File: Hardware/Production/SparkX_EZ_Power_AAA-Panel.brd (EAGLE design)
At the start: 187.2 x 136.7 mm, 1236 parts, among them J10 AVR_SPI_PROG_3X2TESTPOINTS, J12 AVR_SPI_PROG_3X2TESTPOINTS, J14 AVR_SPI_PROG_3X2TESTPOINTS, J16 AVR_SPI_PROG_3X2TESTPOINTS, J18 AVR_SPI_PROG_3X2TESTPOINTS, J20 AVR_SPI_PROG_3X2TESTPOINTS, J22 AVR_SPI_PROG_3X2TESTPOINTS, J24 AVR_SPI_PROG_3X2TESTPOINTS, J26 AVR_SPI_PROG_3X2TESTPOINTS, J28 AVR_SPI_PROG_3X2TESTPOINTS, J3 AVR_SPI_PROG_3X2TESTPOINTS, J30 AVR_SPI_PROG_3X2TESTPOINTS, J32 AVR_SPI_PROG_3X2TESTPOINTS, J34 AVR_SPI_PROG_3X2TESTPOINTS, J36 AVR_SPI_PROG_3X2TESTPOINTS, J38 AVR_SPI_PROG_3X2TESTPOINTS, J4 AVR_SPI_PROG_3X2TESTPOINTS, J40 AVR_SPI_PROG_3X2TESTPOINTS, J42 AVR_SPI_PROG_3X2TESTPOINTS, J44 AVR_SPI_PROG_3X2TESTPOINTS, J46 AVR_SPI_PROG_3X2TESTPOINTS, J48 AVR_SPI_PROG_3X2TESTPOINTS, J50 AVR_SPI_PROG_3X2TESTPOINTS, J52 AVR_SPI_PROG_3X2TESTPOINTS, J54 AVR_SPI_PROG_3X2TESTPOINTS, J56 AVR_SPI_PROG_3X2TESTPOINTS, J58 AVR_SPI_PROG_3X2TESTPOINTS, J6 AVR_SPI_PROG_3X2TESTPOINTS, J60 AVR_SPI_PROG_3X2TESTPOINTS, J8 AVR_SPI_PROG_3X2TESTPOINTS, U1 ATTINY43_QFN20, U10 TPS61200, U11 ATTINY43_QFN20, U12 TPS61200, U13 ATTINY43_QFN20, U14 TPS61200, U15 ATTINY43_QFN20, U16 TPS61200, U17 ATTINY43_QFN20, U18 TPS61200, U19 ATTINY43_QFN20, U2 TPS61200, U20 TPS61200, U21 ATTINY43_QFN20, U22 TPS61200, U23 ATTINY43_QFN20, U24 TPS61200, U25 ATTINY43_QFN20, U26 TPS61200, U27 ATTINY43_QFN20, U28 TPS61200, U29 ATTINY43_QFN20, U3 ATTINY43_QFN20, U30 TPS61200, U31 ATTINY43_QFN20, U32 TPS61200, U33 ATTINY43_QFN20, U34 TPS61200, U35 ATTINY43_QFN20, U36 TPS61200, U37 ATTINY43_QFN20, U38 TPS61200, U39 ATTINY43_QFN20, U4 TPS61200, U40 TPS61200, U41 ATTINY43_QFN20, U42 TPS61200, U43 ATTINY43_QFN20, U44 TPS61200, U45 ATTINY43_QFN20, U46 TPS61200, U47 ATTINY43_QFN20, U48 TPS61200, U49 ATTINY43_QFN20, U5 ATTINY43_QFN20, U50 TPS61200, U51 ATTINY43_QFN20, U52 TPS61200, U53 ATTINY43_QFN20, U54 TPS61200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

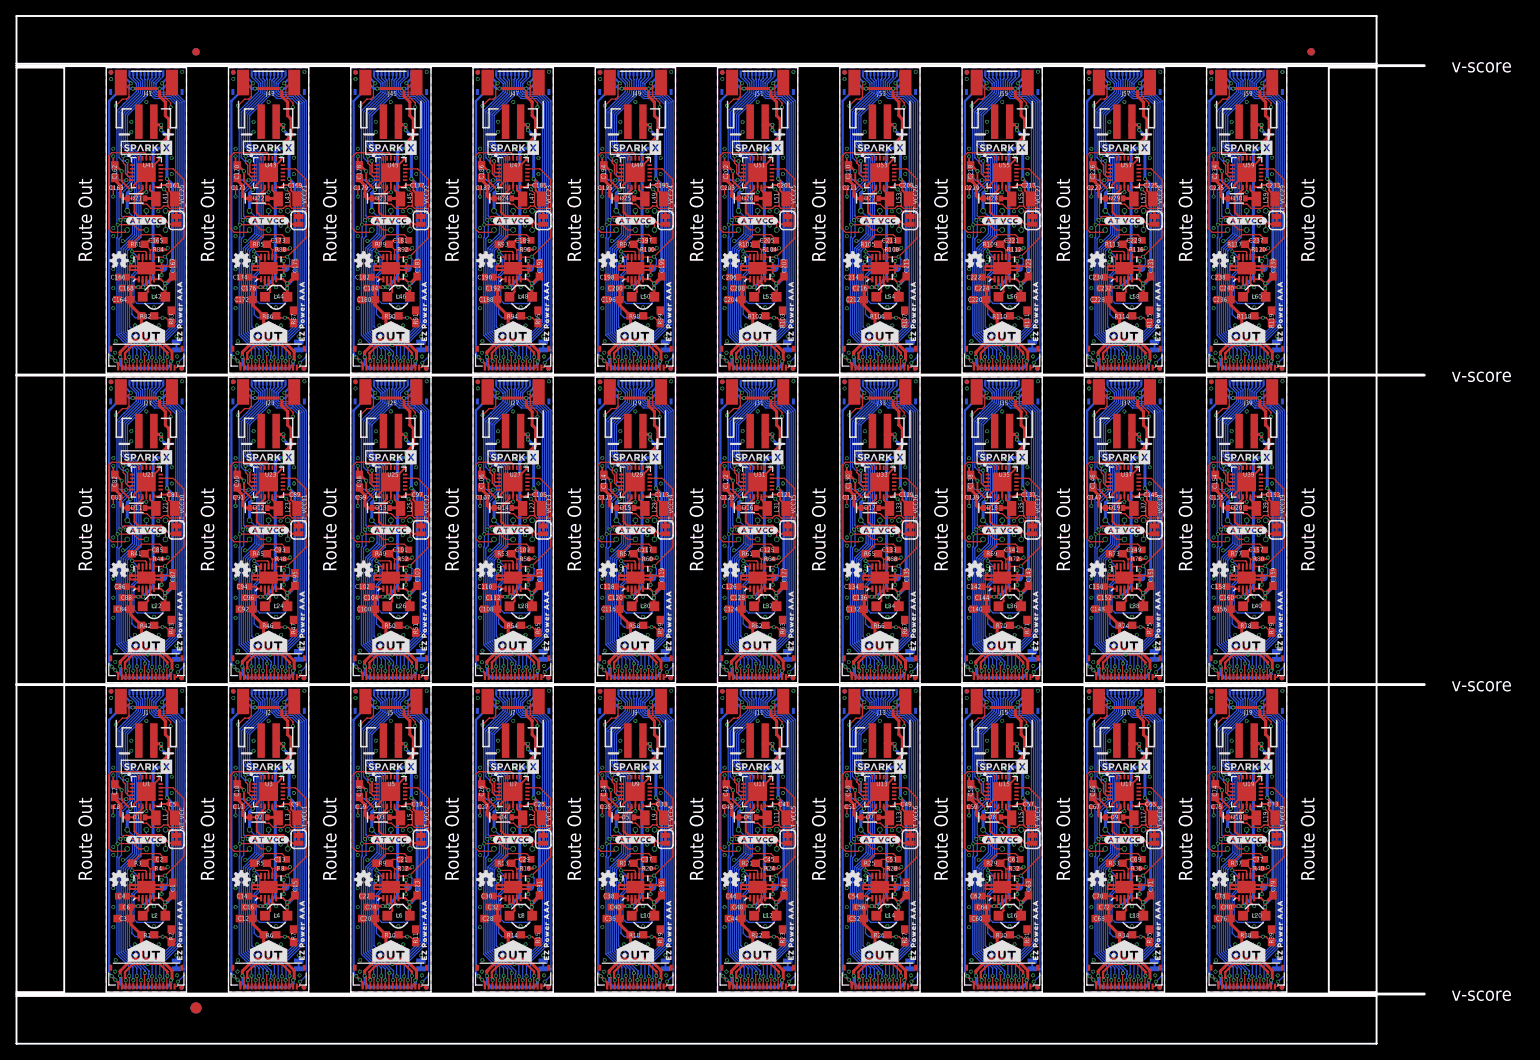
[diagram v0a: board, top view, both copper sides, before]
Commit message: Post-review updates
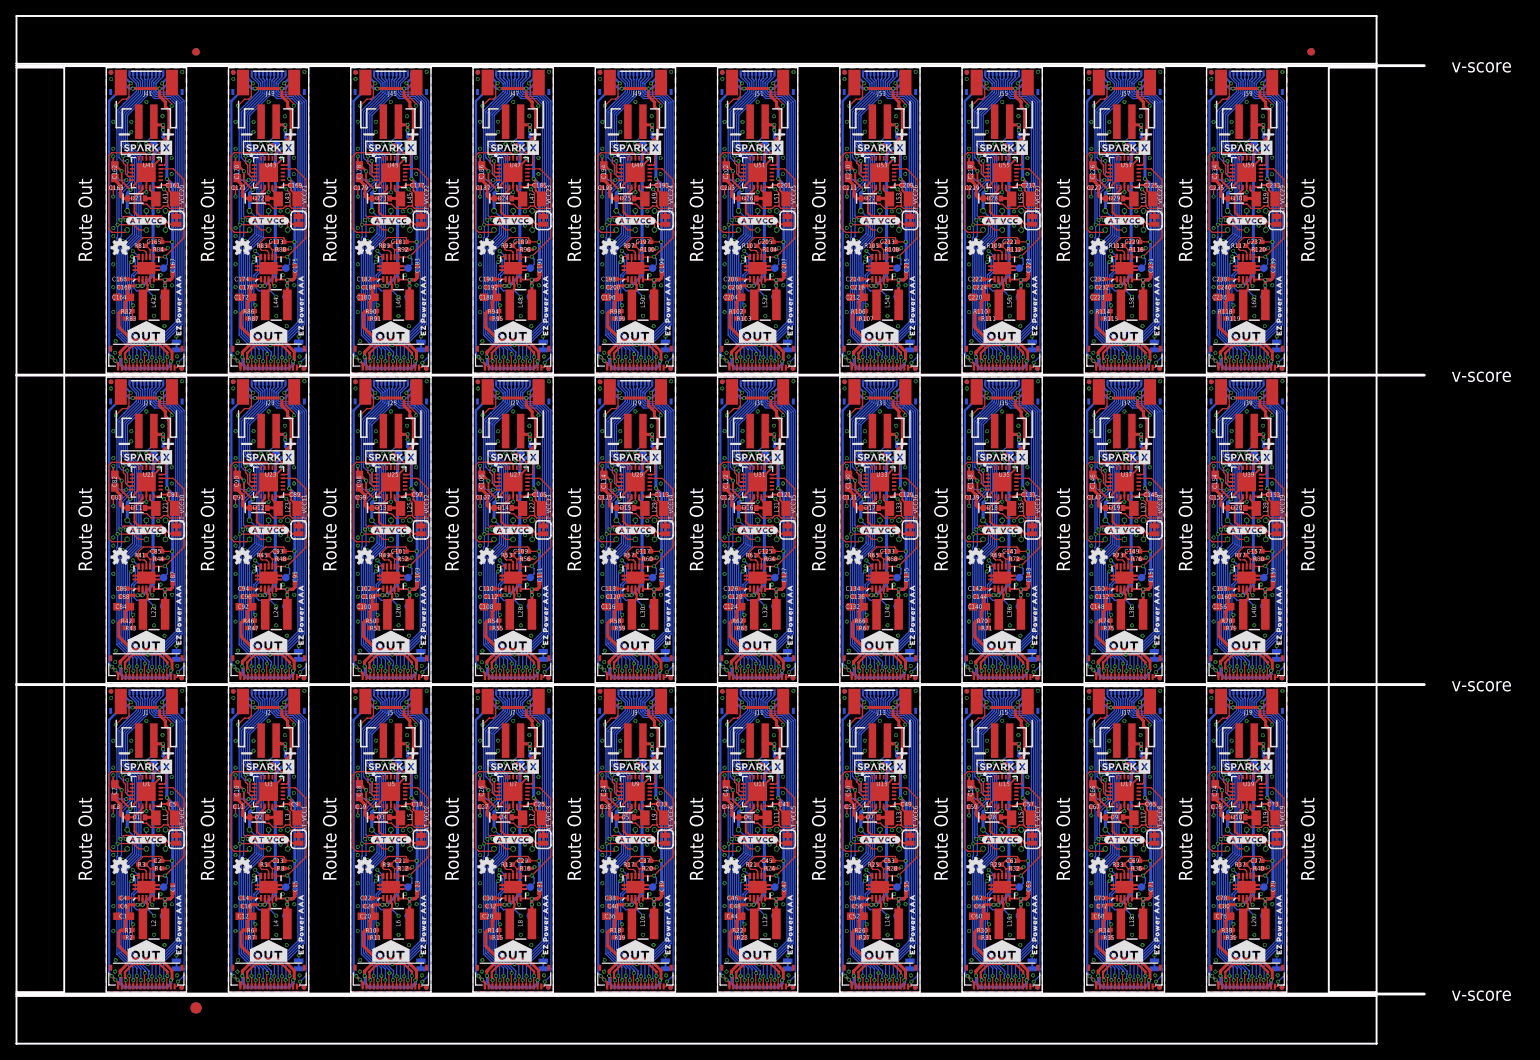
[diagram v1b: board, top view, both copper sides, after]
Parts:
- added RXD, RXD1, RXD10, RXD11, RXD12, RXD13, RXD14, RXD15, RXD16, RXD17, RXD18, RXD19, RXD2, RXD20, RXD21, RXD22, RXD23, RXD24, RXD25, RXD26, RXD27, RXD28, RXD29, RXD3, RXD4, RXD5, RXD6, RXD7, RXD8, RXD9, TXD, TXD1, TXD10, TXD11, TXD12, TXD13, TXD14, TXD15, TXD16, TXD17, TXD18, TXD19, TXD2, TXD20, TXD21, TXD22, TXD23, TXD24, TXD25, TXD26, TXD27, TXD28, TXD29, TXD3, TXD4, TXD5, TXD6, TXD7, TXD8, TXD9: TEST-POINT3X4, SparkFun-Connectors:PAD.03X.04
- added U$301, U$303, U$313, U$315, U$325, U$327, U$337, U$339, U$349, U$351: SPARKX-LOGO3, SparkX:SPARKX-SMALL
- added U$302, U$314, U$326, U$338, U$350: (no value), output:#OUT#0
- added U$304, U$316, U$328, U$340, U$352: (no value), output:#IN#0
- added U$305, U$317, U$329, U$341, U$353: (no value), output:#VIN#0
- added U$306, U$318, U$330, U$342, U$354: (no value), output:#3V3_EN#0
- added U$307, U$319, U$331, U$343, U$355: (no value), output:#PROC_PWR#0
- added U$308, U$320, U$332, U$344, U$356: (no value), output:#AT_VCC#0
- added U$309, U$310, U$321, U$322, U$333, U$334, U$345, U$346, U$357, U$358: (no value), output:EZ_POWER_AAA0
- added U$311, U$323, U$335, U$347, U$359: (no value), output:#TXD#0
- added U$312, U$324, U$336, U$348, U$360: (no value), output:#RXD#0
- C1, C103, C111, C119, C127, C135, C143, C15, C151, C159, C167, C175, C183, C191, C199, C207, C215, C223, C23, C231, C239, C31, C39, C47, C55, C63, C71, C79, C87, C95: device SparkFun-Capacitors:0603 -> SparkFun-Capacitors:0402-TIGHT
- C101, C102, C104, C109, C110, C112, C117, C118, C120, C125, C126, C128, C13, C133, C134, C136, C14, C141, C142, C144, C149, C150, C152, C157, C158, C16, C160, C165, C166, C168, C173, C174, C176, C181, C182, C184, C189, C190, C192, C197, C198, C2, C200, C205, C206, C208, C21, C213, C214, C216, C22, C221, C222, C224, C229, C230, C232, C237, C238, C24, C240, C29, C30, C32, C37, C38, C4, C40, C45, C46, C48, C53, C54, C56, C6, C61, C62, C64, C69, C70, C72, C77, C78, C80, C85, C86, C88, C93, C94, C96: device SparkFun-Capacitors:0402 -> SparkFun-Capacitors:0402-TIGHT
- L10, L12, L14, L16, L18, L2, L20, L22, L24, L26, L28, L30, L32, L34, L36, L38, L4, L40, L42, L44, L46, L48, L50, L52, L54, L56, L58, L6, L60, L8: value 4.7uH, 1.2A -> 4.7μH; device SparkFun:CDRH2D09 -> SparkFun-Coils:INDUCTOR_4X4MM
- R1, R10, R101, R102, R103, R105, R106, R107, R109, R11, R110, R111, R113, R114, R115, R117, R118, R119, R13, R14, R15, R17, R18, R19, R2, R21, R22, R23, R25, R26, R27, R29, R3, R30, R31, R33, R34, R35, R37, R38, R39, R41, R42, R43, R45, R46, R47, R49, R5, R50, R51, R53, R54, R55, R57, R58, R59, R6, R61, R62, R63, R65, R66, R67, R69, R7, R70, R71, R73, R74, R75, R77, R78, R79, R81, R82, R83, R85, R86, R87, R89, R9, R90, R91, R93, R94, R95, R97, R98, R99: device SparkFun-Resistors:0603 -> New-Parts_SparkFun-Resistors:0402-TIGHT
- U$100, U$160, U$220, U$280, U$40: device output:EZ_POWER_AAA0 -> output:#IN#0
- U$101, U$113, U$161, U$173, U$221, U$233, U$281, U$293, U$41, U$53: value SPARKX-LOGO3 -> (none); device SparkX:SPARKX-SMALL -> output:#VIN#0
- U$102, U$162, U$222, U$282, U$42: device output:#OUT#0 -> output:#3V3_EN#0
- U$103, U$151, U$163, U$211, U$223, U$271, U$283, U$31, U$43, U$91: value SPARKX-LOGO3 -> (none); device SparkX:SPARKX-SMALL -> output:#PROC_PWR#0
- U$104, U$164, U$224, U$284, U$44: device output:#IN#0 -> output:#AT_VCC#0
- U$105, U$165, U$225, U$285, U$45: device output:#VIN#0 -> output:EZ_POWER_AAA0
- U$106, U$166, U$226, U$286, U$46: device output:#3V3_EN#0 -> output:EZ_POWER_AAA0
- U$107, U$167, U$227, U$287, U$47: device output:#PROC_PWR#0 -> output:#TXD#0
- U$108, U$168, U$228, U$288, U$48: device output:#AT_VCC#0 -> output:#RXD#0
- U$109, U$159, U$169, U$219, U$229, U$279, U$289, U$39, U$49, U$99: value (none) -> SPARKX-LOGO3; device output:EZ_POWER_AAA0 -> SparkX:SPARKX-SMALL
- U$11, U$134, U$194, U$254, U$74: device output:#IN#0 -> output:#OUT#0
- U$110, U$170, U$230, U$290, U$50: device output:EZ_POWER_AAA0 -> output:#OUT#0
- U$112, U$172, U$232, U$292, U$52: device output:#OUT#0 -> output:#IN#0
- U$114, U$174, U$234, U$294, U$54: device output:#IN#0 -> output:#3V3_EN#0
- U$115, U$175, U$235, U$295, U$55: device output:#VIN#0 -> output:#PROC_PWR#0
- U$116, U$176, U$236, U$296, U$56: device output:#3V3_EN#0 -> output:#AT_VCC#0
- U$117, U$177, U$237, U$297, U$57: device output:#PROC_PWR#0 -> output:EZ_POWER_AAA0
- U$118, U$178, U$238, U$298, U$58: device output:#AT_VCC#0 -> output:EZ_POWER_AAA0
- U$119, U$179, U$239, U$299, U$59: device output:EZ_POWER_AAA0 -> output:#TXD#0
- U$120, U$180, U$240, U$300, U$60: device output:EZ_POWER_AAA0 -> output:#RXD#0
- U$131, U$143, U$191, U$203, U$23, U$251, U$263, U$4, U$71, U$83: value SPARKX-LOGO3 -> (none); device SparkX:SPARKX-SMALL -> output:#TXD#0
- U$132, U$192, U$252, U$72, U$9: device output:#OUT#0 -> output:#RXD#0
- U$135, U$14, U$145, U$195, U$205, U$25, U$255, U$265, U$75, U$85: value (none) -> SPARKX-LOGO3; device output:#VIN#0 -> SparkX:SPARKX-SMALL
- U$136, U$15, U$196, U$256, U$76: device output:#3V3_EN#0 -> output:#IN#0
- U$137, U$16, U$197, U$257, U$77: device output:#PROC_PWR#0 -> output:#VIN#0
- U$138, U$17, U$198, U$258, U$78: device output:#AT_VCC#0 -> output:#3V3_EN#0
- U$139, U$18, U$199, U$259, U$79: device output:EZ_POWER_AAA0 -> output:#PROC_PWR#0
- U$140, U$19, U$200, U$260, U$80: device output:EZ_POWER_AAA0 -> output:#AT_VCC#0
- U$141, U$153, U$201, U$21, U$213, U$261, U$273, U$33, U$81, U$93: value SPARKX-LOGO3 -> (none); device SparkX:SPARKX-SMALL -> output:EZ_POWER_AAA0
- U$142, U$202, U$22, U$262, U$82: device output:#OUT#0 -> output:EZ_POWER_AAA0
- U$144, U$204, U$24, U$264, U$84: device output:#IN#0 -> output:#RXD#0
- U$146, U$206, U$26, U$266, U$86: device output:#3V3_EN#0 -> output:#OUT#0
- U$147, U$157, U$207, U$217, U$267, U$27, U$277, U$37, U$87, U$97: value (none) -> SPARKX-LOGO3; device output:#PROC_PWR#0 -> SparkX:SPARKX-SMALL
- U$148, U$208, U$268, U$28, U$88: device output:#AT_VCC#0 -> output:#IN#0
- U$149, U$209, U$269, U$29, U$89: device output:EZ_POWER_AAA0 -> output:#VIN#0
- U$150, U$210, U$270, U$30, U$90: device output:EZ_POWER_AAA0 -> output:#3V3_EN#0
- U$152, U$212, U$272, U$32, U$92: device output:#OUT#0 -> output:#AT_VCC#0
- U$154, U$214, U$274, U$34, U$94: device output:#IN#0 -> output:EZ_POWER_AAA0
- U$155, U$215, U$275, U$35, U$95: device output:#VIN#0 -> output:#TXD#0
- U$156, U$216, U$276, U$36, U$96: device output:#3V3_EN#0 -> output:#RXD#0
- U$158, U$218, U$278, U$38, U$98: device output:#AT_VCC#0 -> output:#OUT#0
- U10, U12, U14, U16, U18, U2, U20, U22, U24, U26, U28, U30, U32, U34, U36, U38, U4, U40, U42, U44, U46, U48, U50, U52, U54, U56, U58, U6, U60, U8: device SparkFun:QFN-10_PAD -> SparkFun-IC-Power:QFN-10_PAD
- moved U$110 159.3 mm to (151.6, 4.89), flipped to the top
- moved U$105 150.5 mm to (139.7, 9.02), flipped to the top, turned to 90 degrees
- moved U$115 148.2 mm to (150.7, 3.75)
- moved U$103 145.3 mm to (134.5, 3.75)
- moved U$101 143.7 mm to (135.4, 10.2), flipped to the bottom
- moved U$113 143.4 mm to (151.7, 10.2)
- moved U$109 143.2 mm to (151.6, 30.0), turned to 0 degrees
- moved U$114 143.2 mm to (150.7, 14.0)
- moved U$104 141.5 mm to (135.4, 20.3), flipped to the top
- moved U$117 140.0 mm to (156.0, 9.02), flipped to the top, turned to 90 degrees
- moved U$111 137.0 mm to (151.6, 27.9), flipped to the bottom
- moved U$116 135.6 mm to (151.6, 20.3), flipped to the top
- moved U$118 134.8 mm to (151.6, 26.0), flipped to the bottom
- moved U$106 134.2 mm to (135.4, 26.0)
- moved U$120 134.0 mm to (150.3, 30.5)
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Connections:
- new net RXD: RXD.1, U1.16
- new net RXD1: RXD1.1, U3.16
- new net RXD10: RXD10.1, U21.16
- new net RXD11: RXD11.1, U23.16
- new net RXD12: RXD12.1, U25.16
- new net RXD13: RXD13.1, U27.16
- new net RXD14: RXD14.1, U29.16
- new net RXD15: RXD15.1, U31.16
- new net RXD16: RXD16.1, U33.16
- new net RXD17: RXD17.1, U35.16
- new net RXD18: RXD18.1, U37.16
- new net RXD19: RXD19.1, U39.16
- new net RXD2: RXD2.1, U5.16
- new net RXD20: RXD20.1, U41.16
- new net RXD21: RXD21.1, U43.16
- new net RXD22: RXD22.1, U45.16
- new net RXD23: RXD23.1, U47.16
- new net RXD24: RXD24.1, U49.16
- new net RXD25: RXD25.1, U51.16
- new net RXD26: RXD26.1, U53.16
- new net RXD27: RXD27.1, U55.16
- new net RXD28: RXD28.1, U57.16
- new net RXD29: RXD29.1, U59.16
- new net RXD3: RXD3.1, U7.16
- new net RXD4: RXD4.1, U9.16
- new net RXD5: RXD5.1, U11.16
- new net RXD6: RXD6.1, U13.16
- new net RXD7: RXD7.1, U15.16
- new net RXD8: RXD8.1, U17.16
- new net RXD9: RXD9.1, U19.16
- new net TXD: TXD.1, U1.15
- new net TXD1: TXD1.1, U3.15
- new net TXD10: TXD10.1, U21.15
- new net TXD11: TXD11.1, U23.15
- new net TXD12: TXD12.1, U25.15
- new net TXD13: TXD13.1, U27.15
- new net TXD14: TXD14.1, U29.15
- new net TXD15: TXD15.1, U31.15
- new net TXD16: TXD16.1, U33.15
- new net TXD17: TXD17.1, U35.15
- new net TXD18: TXD18.1, U37.15
- new net TXD19: TXD19.1, U39.15
- new net TXD2: TXD2.1, U5.15
- new net TXD20: TXD20.1, U41.15
- new net TXD21: TXD21.1, U43.15
- new net TXD22: TXD22.1, U45.15
- new net TXD23: TXD23.1, U47.15
- new net TXD24: TXD24.1, U49.15
- new net TXD25: TXD25.1, U51.15
- new net TXD26: TXD26.1, U53.15
- new net TXD27: TXD27.1, U55.15
- new net TXD28: TXD28.1, U57.15
- new net TXD29: TXD29.1, U59.15
- new net TXD3: TXD3.1, U7.15
- new net TXD4: TXD4.1, U9.15
- new net TXD5: TXD5.1, U11.15
- new net TXD6: TXD6.1, U13.15
- new net TXD7: TXD7.1, U15.15
- new net TXD8: TXD8.1, U17.15
- new net TXD9: TXD9.1, U19.15
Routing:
- net VIN29: track 57.7 -> 46.2 mm
- net VIN18: track 57.7 -> 46.2 mm
- net VIN9: track 57.7 -> 46.2 mm
- net VIN8: track 57.7 -> 46.2 mm
- net VIN28: track 57.7 -> 46.2 mm
- net VIN19: track 57.7 -> 46.2 mm
- net VIN23: track 57.7 -> 46.2 mm
- net VIN: track 57.7 -> 46.2 mm
- net VIN22: track 57.7 -> 46.2 mm
- net VIN3: track 57.7 -> 46.2 mm
- net VIN13: track 57.7 -> 46.2 mm
- net VIN1: track 57.7 -> 46.2 mm
- net VIN21: track 57.7 -> 46.2 mm
- net VIN20: track 57.7 -> 46.2 mm
- net VIN11: track 57.7 -> 46.2 mm
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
